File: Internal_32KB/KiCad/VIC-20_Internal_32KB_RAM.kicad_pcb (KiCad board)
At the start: 2 copper layers, 66 x 62.2 mm, 17 parts, among them J1 BLK Decoder, J2 RAM Decoder, J3 Disable/Enable Switch, J4 UD4, J5 UE4, U1 74HCT138, U2 74HCT138, U3 74HCT10, U4 74HCT30, U5 74HCT157, U6 62256

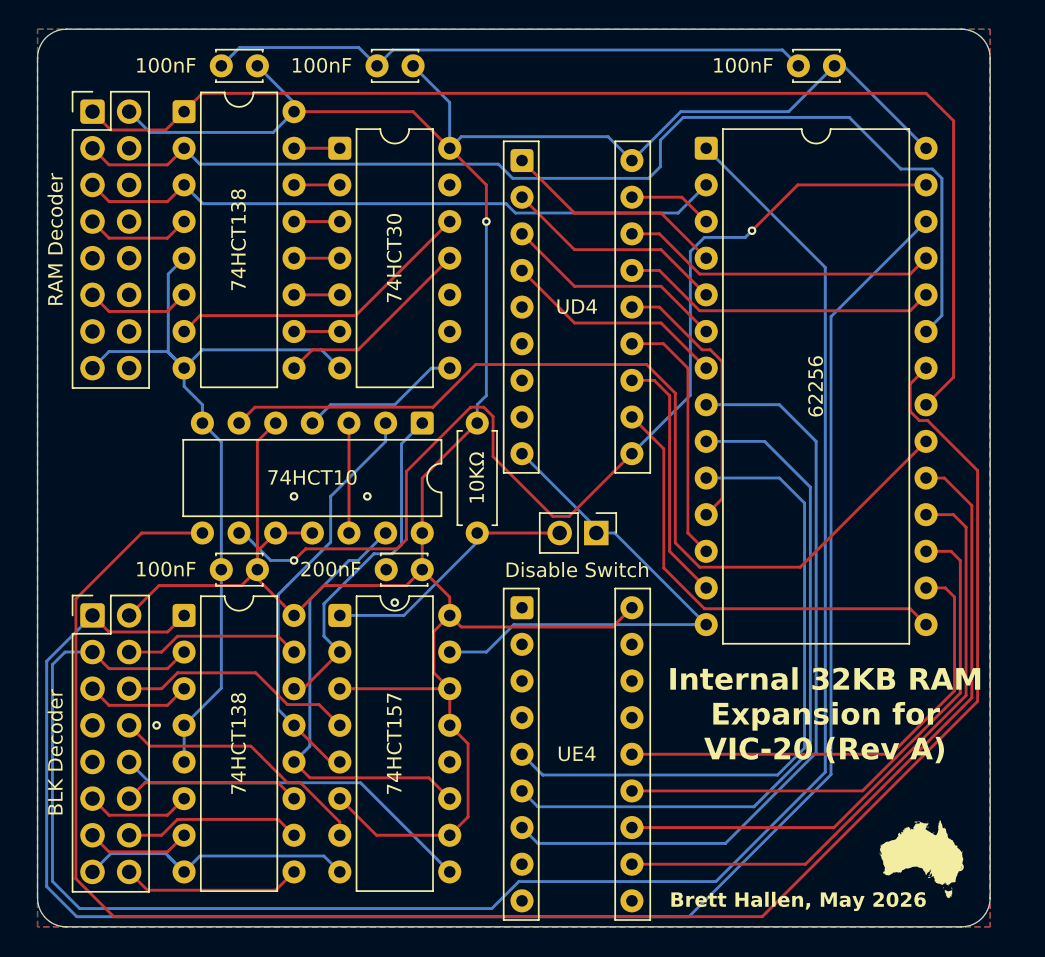
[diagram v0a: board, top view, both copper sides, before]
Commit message: Further design corrections
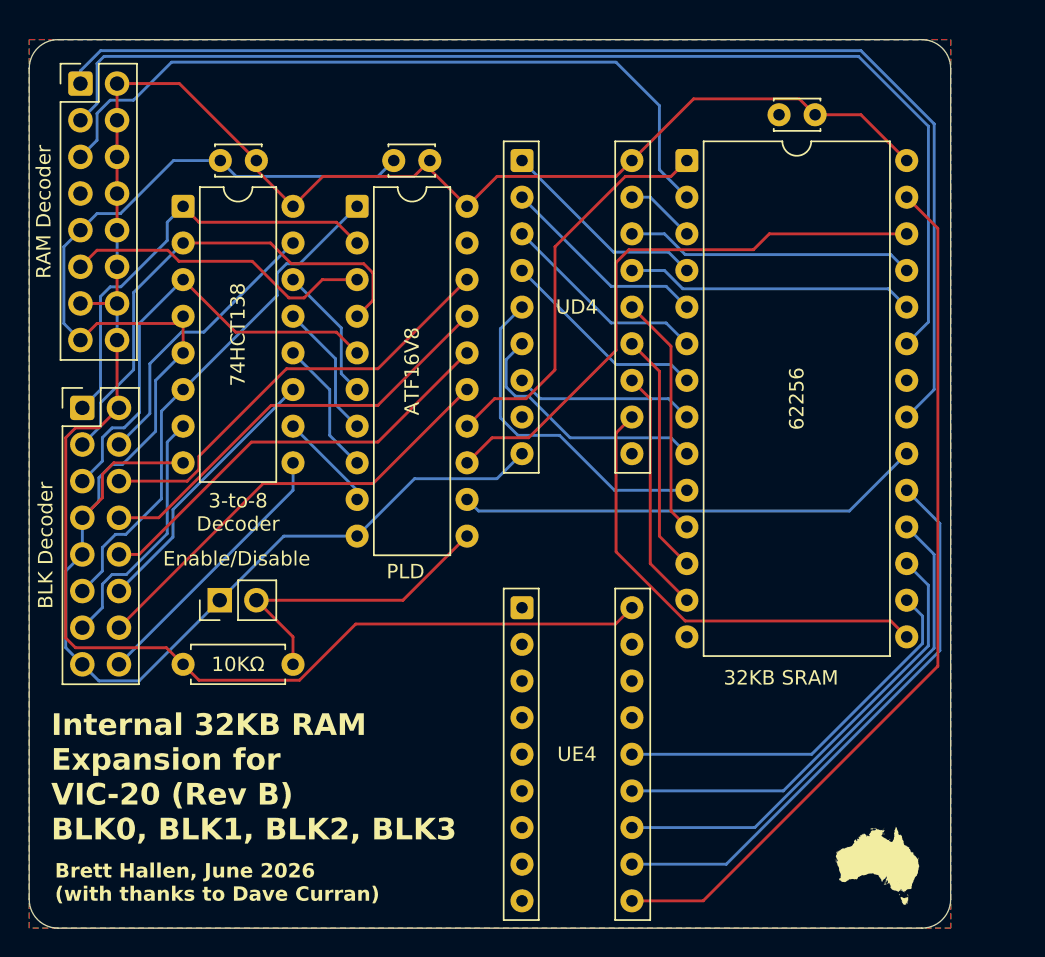
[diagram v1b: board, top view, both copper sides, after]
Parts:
- removed C4: 100nF, Capacitor_THT:C_Disc_D3.0mm_W2.0mm_P2.50mm
- removed C5: 200nF, Capacitor_THT:C_Disc_D3.0mm_W2.0mm_P2.50mm
- removed the U2 at (76.7, 37.2)
- removed the U3 at (93.2, 58.8)
- removed U4: 74HCT30, Package_DIP:DIP-14_W7.62mm
- removed U5: 74HCT157, Package_DIP:DIP-16_W7.62mm
- added U1: ATF16V8, Package_DIP:DIP-20_W7.62mm, F.Cu at (88.7, 43.8)
- moved U2 28.4 mm to (76.6, 43.8)
- moved J5 26.5 mm to (79.2, 71.1), turned to 90 degrees
- moved R1 26.4 mm to (76.6, 75.6), turned to 0 degrees
- moved J4 14.4 mm to (69.7, 57.8)
- moved C1 13.6 mm to (93.7, 40.6)
- moved C2 12.7 mm to (81.7, 40.6)
- moved C3 3.65 mm to (120.5, 37.5)
- moved J3 2.12 mm to (69.5, 35.3)
- moved U3 1.59 mm to (111.6, 40.6)
- renumbered J4 to J1, J5 to J2, J2 to J3, J1 to J4, J3 to J5, U1 to U2, U6 to U3
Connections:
- net /BD0 renamed BD0
- net /BD1 renamed BD1
- net /BD2 renamed BD2
- net /BD3 renamed BD3
- net /BD4 renamed BD4
- net /BD5 renamed BD5
- net /BD6 renamed BD6
- net /BD7 renamed BD7
- net /CA15 renamed CA15
- net /SΦ2/G1 renamed SΦ2
- net /VA10 renamed VA10
- net /VA11 renamed VA11
- net /VA12 renamed VA12
- net /VA3 renamed VA3
- net /VA4 renamed VA4
- net /VA5 renamed VA5
- net /VA6 renamed VA6
- net /VA7 renamed VA7
- net /VA8 renamed VA8
- net /VA9 renamed VA9
- net /~{BLK0} renamed ~{BLK0}
- net /~{BLK4} renamed ~{BLK4}
- net /~{BLK6} renamed ~{BLK6}
- net /~{BLK7} renamed ~{BLK7}
- net Net-(J3-Pin_2) renamed ENABLE
- J1 pad 10: /VR/~{W} -> unconnected-(J1-Pin_10-Pad10)
- J1 pad 5: unconnected-(J4-Pin_5-Pad5) -> VA0
- J1 pad 6: unconnected-(J4-Pin_6-Pad6) -> VA1
- J1 pad 7: unconnected-(J4-Pin_7-Pad7) -> VA2
- J2 pad 10: unconnected-(J5-Pin_10-Pad10) -> VR/~{W}
- J2 pad 5: /VA0 -> unconnected-(J2-Pin_5-Pad5)
- J2 pad 6: /VA1 -> unconnected-(J2-Pin_6-Pad6)
- J2 pad 7: /VA2 -> unconnected-(J2-Pin_7-Pad7)
- J3 pad 10: unconnected-(J2-Pin_10-Pad10) -> +5V
- J3 pad 11: unconnected-(J2-Pin_11-Pad11) -> +5V
- J3 pad 12: unconnected-(J2-Pin_12-Pad12) -> +5V
- J3 pad 13: unconnected-(J2-Pin_13-Pad13) -> +5V
- J3 pad 14: unconnected-(J2-Pin_14-Pad14) -> +5V
- J3 pad 15: unconnected-(J2-Pin_15-Pad15) (its old number) -> +5V
- J3 pad 4: /~{BLK0}/~{G2A} -> unconnected-(J3-Pin_4-Pad4)
- J3 pad 5: unconnected-(J2-Pin_5-Pad5) -> GND
- J3 pad 6: /VA13/G1 -> VA13
- J3 pad 7: unconnected-(J2-Pin_7-Pad7) -> +5V
- J3 pad 9: unconnected-(J2-Pin_9-Pad9) -> +5V
- J4 pad 1: /CA13 -> CA13
- J4 pad 10: /~{BLK5} -> ~{BLK5_OUT}
- J4 pad 12: /~{BLK3_{OUT}} -> ~{BLK3_OUT}
- J4 pad 13: /~{BLK2_{OUT}} -> ~{BLK2_OUT}
- J4 pad 14: /~{BLK1_{OUT}} -> ~{BLK1_OUT}
- J4 pad 2: /CA14 -> CA14
- J4 pad 4: unconnected-(J1-Pin_4-Pad4) -> GND
- J4 pad 5: unconnected-(J1-Pin_5-Pad5) -> GND
- U2 pad 1: /CA13 -> CA13
- U2 pad 10: /~{BLK5} -> ~{BLK5}
- U2 pad 12: /~{BLK3} -> ~{BLK3}
- U2 pad 13: /~{BLK2} -> ~{BLK2}
- U2 pad 14: /~{BLK1} -> ~{BLK1}
- U2 pad 2: /CA14 -> CA14
- U3 pad 1: /CA14 -> RAM_A14
- U3 pad 10: /VA0 -> VA0
- U3 pad 20: /~{CS} -> ~{RAM_CS}
- U3 pad 22: /~{OE} -> GND
- U3 pad 26: /CA13 -> RAM_A13
- U3 pad 27: /VR/~{W} -> VR/~{W}
- U3 pad 8: /VA2 -> VA2
- U3 pad 9: /VA1 -> VA1
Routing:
- net /CA14: track 130.4 -> 0.00 mm
- net /CA13: track 127.8 -> 0.00 mm
- net /~{OE}: track 125.7 -> 0.00 mm
- net /VR/~{W}: track 75.7 -> 0.00 mm, vias 2 -> 0
- net /~{CS}: track 64.8 -> 0.00 mm
- net VR/~{W}: track 0.00 -> 61.4 mm
- net /VA2: track 53.7 -> 0.00 mm
- net /VA1: track 48.8 -> 0.00 mm
- net +5V: track 199.5 -> 152.5 mm, vias 1 -> 0
- net /VA0: track 46.1 -> 0.00 mm
- net GND: track 157.1 -> 116.4 mm, vias 5 -> 0
- net RAM_A13: track 0.00 -> 40.6 mm
- net CA14: track 0.00 -> 34.3 mm
- net ~{RAM_CS}: track 0.00 -> 32.5 mm
- net ~{BLK5_OUT}: track 0.00 -> 31.0 mm
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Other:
- board size 66 x 62.2 mm -> 63.9 x 61.6 mm
- board text added: "10-JUN-2026: Pending testing"
- board text added: "Brett Hallen, June 2026 (with thanks to Dave Curran)"
- board text added: "Enable/Disable"
- board text added: "Internal 32KB RAM Expansion for VIC-20 (Rev B) BLK0, BLK1, BLK2, BLK3"
- board text added: "PLD"
- board text removed: "2114 SRAM Socket"
- board text removed: "26-MAY-2026: Pending testing"
- board text removed: "8-Input NAND Gate"
- board text removed: "Brett Hallen, May 2026"
- board text removed: "Disable Switch"
- board text removed: "Internal 32KB RAM Expansion for VIC-20 (Rev A)"
- board text removed: "Quad 2-Input Multiplexer"
- board text removed: "To/From VIC"
- board text removed: "Triple 3-Input NAND Gate"
